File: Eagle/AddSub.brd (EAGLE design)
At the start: 100 x 80 mm, 238 parts, among them Q1 310mA/60V/1.6Ω, Q10 310mA/60V/1.6Ω, Q100 310mA/60V/1.6Ω, Q101 310mA/60V/1.6Ω, Q102 310mA/60V/1.6Ω, Q103 310mA/60V/1.6Ω, Q104 310mA/60V/1.6Ω, Q105 310mA/60V/1.6Ω, Q106 310mA/60V/1.6Ω, Q107 310mA/60V/1.6Ω, Q108 310mA/60V/1.6Ω, Q109 310mA/60V/1.6Ω, Q11 310mA/60V/1.6Ω, Q110 310mA/60V/1.6Ω, Q111 310mA/60V/1.6Ω, Q112 310mA/60V/1.6Ω, Q113 310mA/60V/1.6Ω, Q114 310mA/60V/1.6Ω, Q115 310mA/60V/1.6Ω, Q116 310mA/60V/1.6Ω, Q117 310mA/60V/1.6Ω, Q118 310mA/60V/1.6Ω, Q119 310mA/60V/1.6Ω, Q12 310mA/60V/1.6Ω, Q120 310mA/60V/1.6Ω, Q121 310mA/60V/1.6Ω, Q122 310mA/60V/1.6Ω, Q123 310mA/60V/1.6Ω, Q124 310mA/60V/1.6Ω, Q125 310mA/60V/1.6Ω, Q126 310mA/60V/1.6Ω, Q127 310mA/60V/1.6Ω, Q128 310mA/60V/1.6Ω, Q129 310mA/60V/1.6Ω, Q13 310mA/60V/1.6Ω, Q130 310mA/60V/1.6Ω, Q131 310mA/60V/1.6Ω, Q132 310mA/60V/1.6Ω, Q133 310mA/60V/1.6Ω, Q14 310mA/60V/1.6Ω, Q141 310mA/60V/1.6Ω, Q142 310mA/60V/1.6Ω, Q143 310mA/60V/1.6Ω, Q144 310mA/60V/1.6Ω, Q145 310mA/60V/1.6Ω, Q146 310mA/60V/1.6Ω, Q147 310mA/60V/1.6Ω, Q148 310mA/60V/1.6Ω, Q149 310mA/60V/1.6Ω, Q15 310mA/60V/1.6Ω, Q150 310mA/60V/1.6Ω, Q155 310mA/60V/1.6Ω, Q156 310mA/60V/1.6Ω, Q157 310mA/60V/1.6Ω, Q158 310mA/60V/1.6Ω, Q159 310mA/60V/1.6Ω, Q16 310mA/60V/1.6Ω, Q163 310mA/60V/1.6Ω, Q164 310mA/60V/1.6Ω, Q165 310mA/60V/1.6Ω, Q166 310mA/60V/1.6Ω, Q167 310mA/60V/1.6Ω, Q168 310mA/60V/1.6Ω, Q169 310mA/60V/1.6Ω, Q17 310mA/60V/1.6Ω, Q177 310mA/60V/1.6Ω, Q178 310mA/60V/1.6Ω, Q179 310mA/60V/1.6Ω, Q18 310mA/60V/1.6Ω, Q180 310mA/60V/1.6Ω, Q181 310mA/60V/1.6Ω, Q182 310mA/60V/1.6Ω, Q183 310mA/60V/1.6Ω, Q19 310mA/60V/1.6Ω, Q2 310mA/60V/1.6Ω, Q20 310mA/60V/1.6Ω, Q21 310mA/60V/1.6Ω, Q22 310mA/60V/1.6Ω, Q23 310mA/60V/1.6Ω, Q24 310mA/60V/1.6Ω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

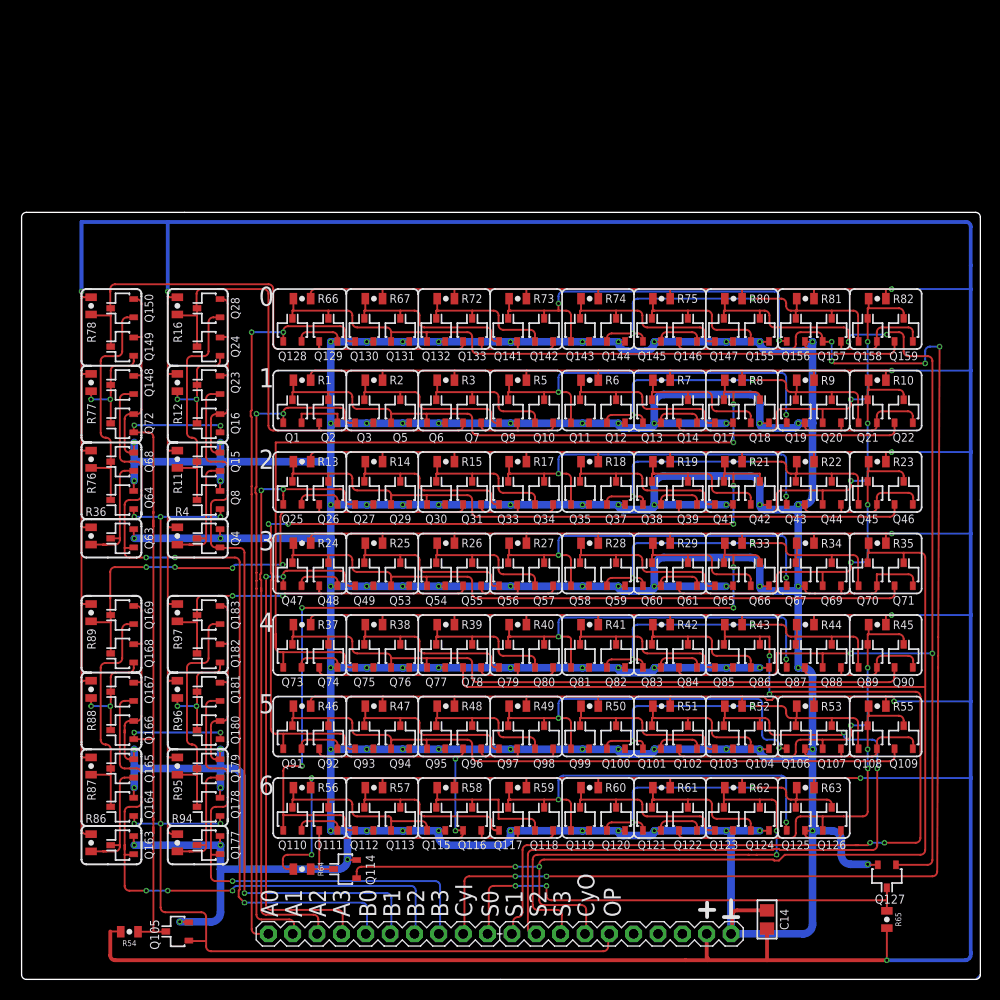
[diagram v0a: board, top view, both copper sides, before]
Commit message: Updated boards with pcb template
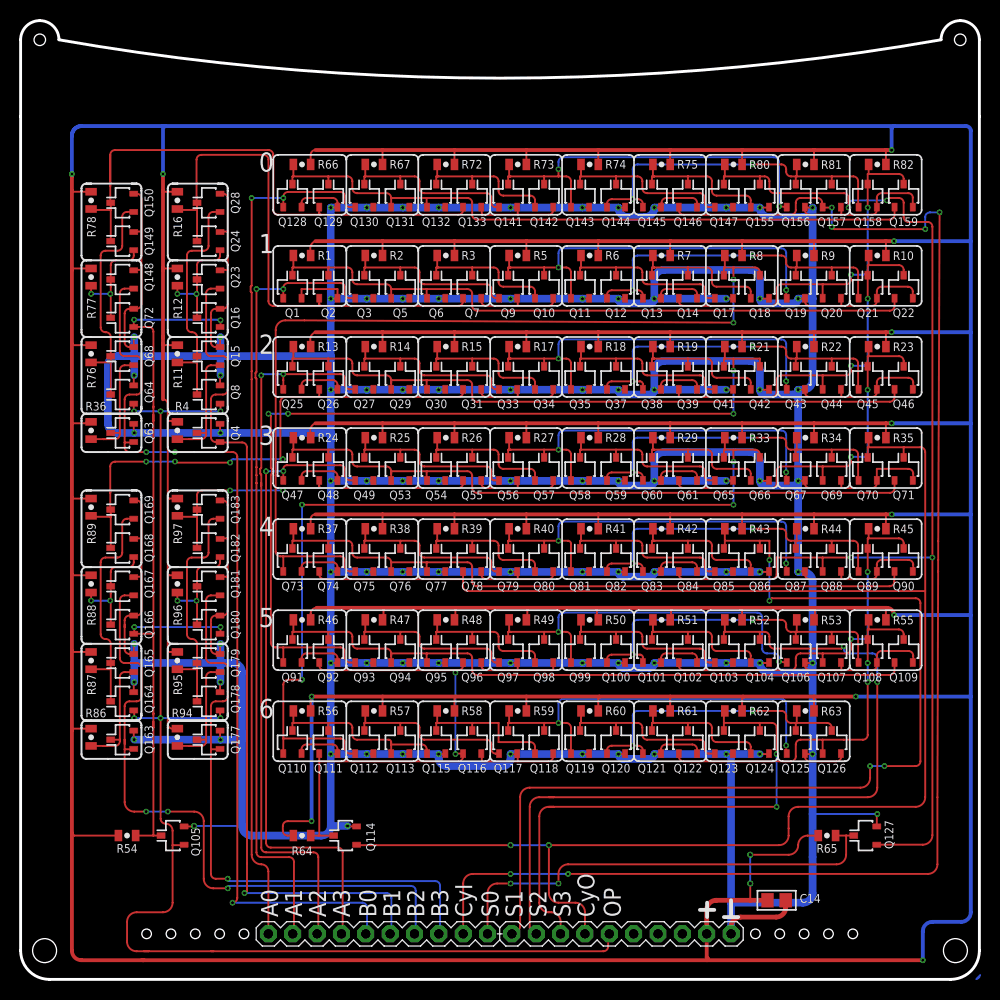
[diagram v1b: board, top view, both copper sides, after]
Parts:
- moved Q128 14.0 mm to (28.2, 81.8)
- moved Q129 14.0 mm to (32.0, 81.8)
- moved Q130 14.0 mm to (35.8, 81.8)
- moved Q131 14.0 mm to (39.5, 81.8)
- moved Q132 14.0 mm to (43.2, 81.8)
- moved Q133 14.0 mm to (47.0, 81.8)
- moved Q141 14.0 mm to (50.8, 81.8)
- moved Q142 14.0 mm to (54.5, 81.8)
- moved Q143 14.0 mm to (58.2, 81.8)
- moved Q144 14.0 mm to (62.0, 81.8)
- moved Q145 14.0 mm to (65.8, 81.8)
- moved Q146 14.0 mm to (69.5, 81.8)
- moved Q147 14.0 mm to (73.2, 81.8)
- moved Q155 14.0 mm to (77.0, 81.8)
- moved Q156 14.0 mm to (80.8, 81.8)
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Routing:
- net VCC: track 975.1 -> 1066.3 mm, vias 12 -> 14
- net GND: track 1034.8 -> 1079.8 mm
- net OP: track 115.8 -> 134.8 mm
- net SUM0': track 116.3 -> 129.9 mm
- net CRYIN: track 143.2 -> 156.8 mm
- net A0: track 77.4 -> 90.6 mm
- net A1: track 70.4 -> 83.4 mm
- net A2: track 64.6 -> 76.6 mm
- net B0: track 85.5 -> 97.4 mm
- net B1: track 78.3 -> 89.6 mm
- net A3: track 56.4 -> 67.4 mm
- net B3: track 52.6 -> 63.5 mm
- net B2: track 60.2 -> 69.4 mm
- net SUM1: track 96.1 -> 105.2 mm
- net SUM2: track 77.3 -> 85.6 mm
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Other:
- board size 100 x 80 mm -> 100 x 100 mm
- board text added: "Adder/ subtractor rev1"
- board text removed: "Addder/ Subtractor rev 1"
